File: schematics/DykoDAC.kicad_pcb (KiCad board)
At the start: 2 copper layers, 99.4 x 100.1 mm, 142 parts, among them J1 AC Input, J2 AudioJack, J3 USB_B, J4 OLED, J5 Debug, J6 Conn_01x05, J7 Conn_01x04, J8 Conn_01x05, J9 Conn_01x04, SW1 PEC09-2120K, U1 LT1762-5, U10 TPA6120A2, U11 PRTR5V0U2X.215, U13 ATSAMD51J20A-A, U2 LM317, U3 LM337, U4 L7805, U5 78L05, U6 LP5907-3.3, U7 LP5907-3.3, U8 CS4398, U9 AD8620, X1 22.5792Mhz, X2 24.576Mhz

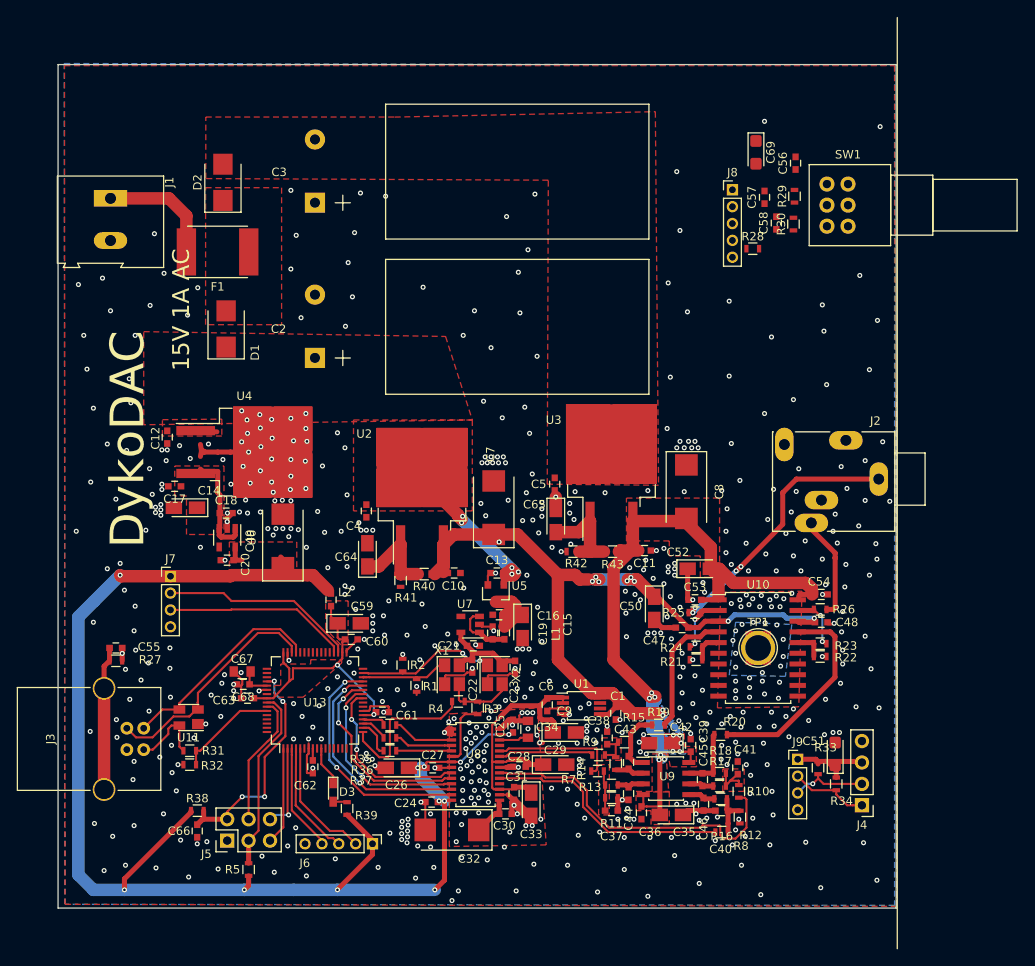
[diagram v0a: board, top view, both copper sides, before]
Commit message: first revision finished
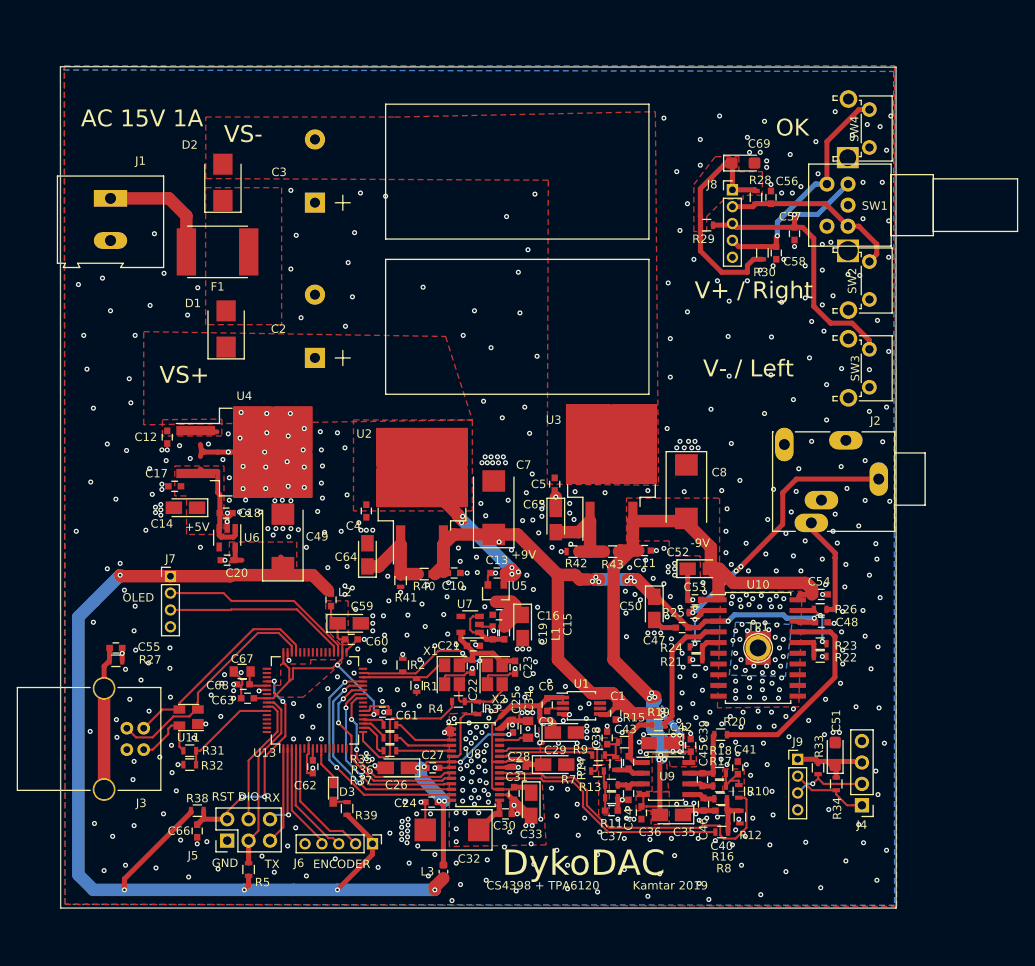
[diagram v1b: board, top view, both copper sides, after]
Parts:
- added L3: Ferrite Bead, Capacitor_SMD:C_0603_1608Metric, F.Cu at (93.5, 135.4)
- added SW2: Button A, Button_Switch_THT:SW_Tactile_SPST_Angled_PTS645Vx58-2LFS, F.Cu at (144.0, 63.0)
- added SW3: Button B, Button_Switch_THT:SW_Tactile_SPST_Angled_PTS645Vx58-2LFS, F.Cu at (144.0, 73.4)
- added SW4: The Button, Button_Switch_THT:SW_Tactile_SPST_Angled_PTS645Vx58-2LFS, F.Cu at (144.0, 45.0)
- SW1: value PEC09-2120K -> EC11B152420G; footprint Potentiometers:Potentiometer_Alps_RK097_Double_Vertical -> kamtar:Potentiometer_Alps_RK097_Dual_Horizontal
- TP1: footprint Connect:1pin -> TestPoint:TestPoint_Plated_Hole_D2.0mm
- moved R29 11.0 mm to (124.7, 58.7), turned to 180 degrees
- moved R28 6.11 mm to (130.6, 55.4), turned to 270 degrees
- moved C57 5.59 mm to (135.1, 59.7), turned to 270 degrees
- moved R30 5.03 mm to (131.3, 62.0)
- moved C56 5.00 mm to (132.3, 55.4), turned to 270 degrees
- moved C58 3.56 mm to (133.0, 62.0)
- moved C69 1.98 mm to (129.0, 51.3), turned to 0 degrees
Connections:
- C24 pad 1: +3V3 -> /DykoDAC_CS4398/3V3_CS
- C25 pad 1: +3V3 -> /DykoDAC_CS4398/3V3_CS
- C26 pad 1: +3V3 -> /DykoDAC_CS4398/3V3_CS
- C27 pad 1: +3V3 -> /DykoDAC_CS4398/3V3_CS
- C56 pad 2: Net-(C56-Pad2) -> /DykoDAC_MCU/BA
- C57 pad 1: Net-(C57-Pad1) -> /DykoDAC_MCU/BB
- C69 pad 1: +3V3 -> /DykoDAC_MCU/3V3_Conn
- J8 pad 2: Net-(C56-Pad2) -> /DykoDAC_MCU/BA
- J8 pad 3: Net-(C57-Pad1) -> /DykoDAC_MCU/BB
- R28 pad 2: Net-(C56-Pad2) -> /DykoDAC_MCU/BA
- R29 pad 1: Net-(C57-Pad1) -> /DykoDAC_MCU/BB
- U8 pad 14: +3V3 -> /DykoDAC_CS4398/3V3_CS
- U8 pad 27: +3V3 -> /DykoDAC_CS4398/3V3_CS
- U8 pad 7: +3V3 -> /DykoDAC_CS4398/3V3_CS
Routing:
- net /DykoDAC_MCU/BB: track 0.00 -> 39.5 mm, vias 0 -> 1
- net +3V3: track 169.8 -> 137.7 mm, vias 11 -> 5
- net /DykoDAC_CS4398/3V3_CS: track 0.00 -> 30.5 mm, vias 0 -> 6
- net /DykoDAC_MCU/3V3_Conn: track 0.00 -> 28.0 mm
- net /DykoDAC_MCU/BTT: track 0.00 -> 27.9 mm, vias 0 -> 1
- net /DykoDAC_MCU/BA: track 0.00 -> 21.9 mm
- net GND: vias 596 -> 703
- added copper zone on F.Cu, net /DykoDAC_MCU/3V3_Conn
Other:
- board size 99.4 x 100.1 mm -> 99.2 x 99.8 mm
- board text added: "+5V"
- board text added: "+9V"
- board text added: "-9V"
- board text added: "AC 15V 1A"
- board text added: "CS4398 + TPA6120"
- board text added: "DIO"
- board text added: "GND"
- board text added: "Kamtar 2019"
- board text added: "OK"
- board text added: "RST"
- board text added: "RX"
- board text added: "TX"
- board text added: "V+ / Right"
- board text added: "V- / Left"
- board text added: "VS+"
- board text added: "VS-"
- board text removed: "15V 1A AC"
- board text removed: "AudioJack"
- board text removed: "POWER JACK"
- board text removed: "USB B"
